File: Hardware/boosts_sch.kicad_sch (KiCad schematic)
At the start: 23 parts, among them IC3 AP2205-W5-7, IC4 TPS61089RNRR

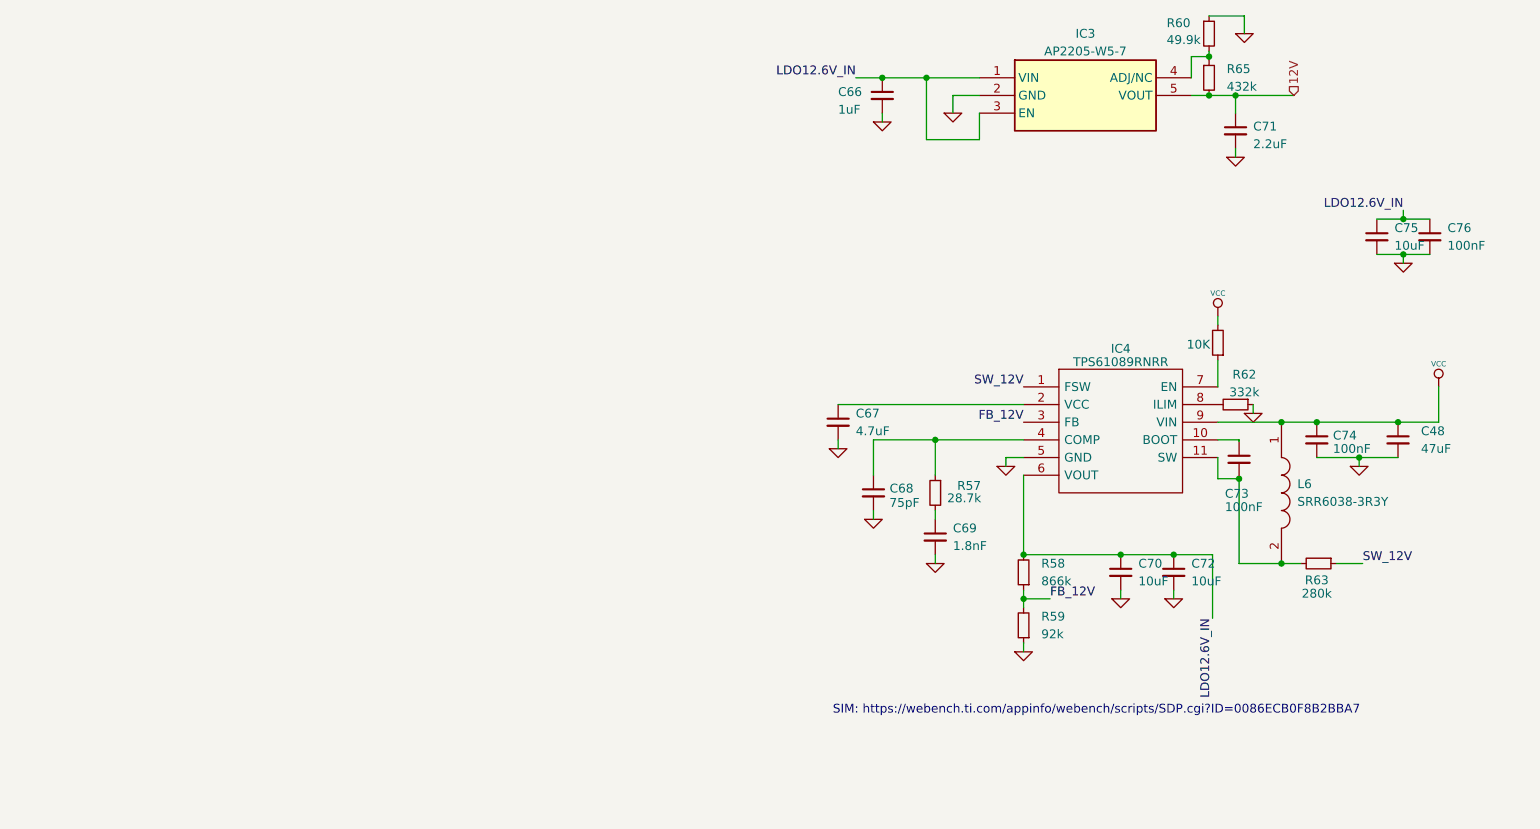
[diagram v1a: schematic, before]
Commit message: changes made post will's review
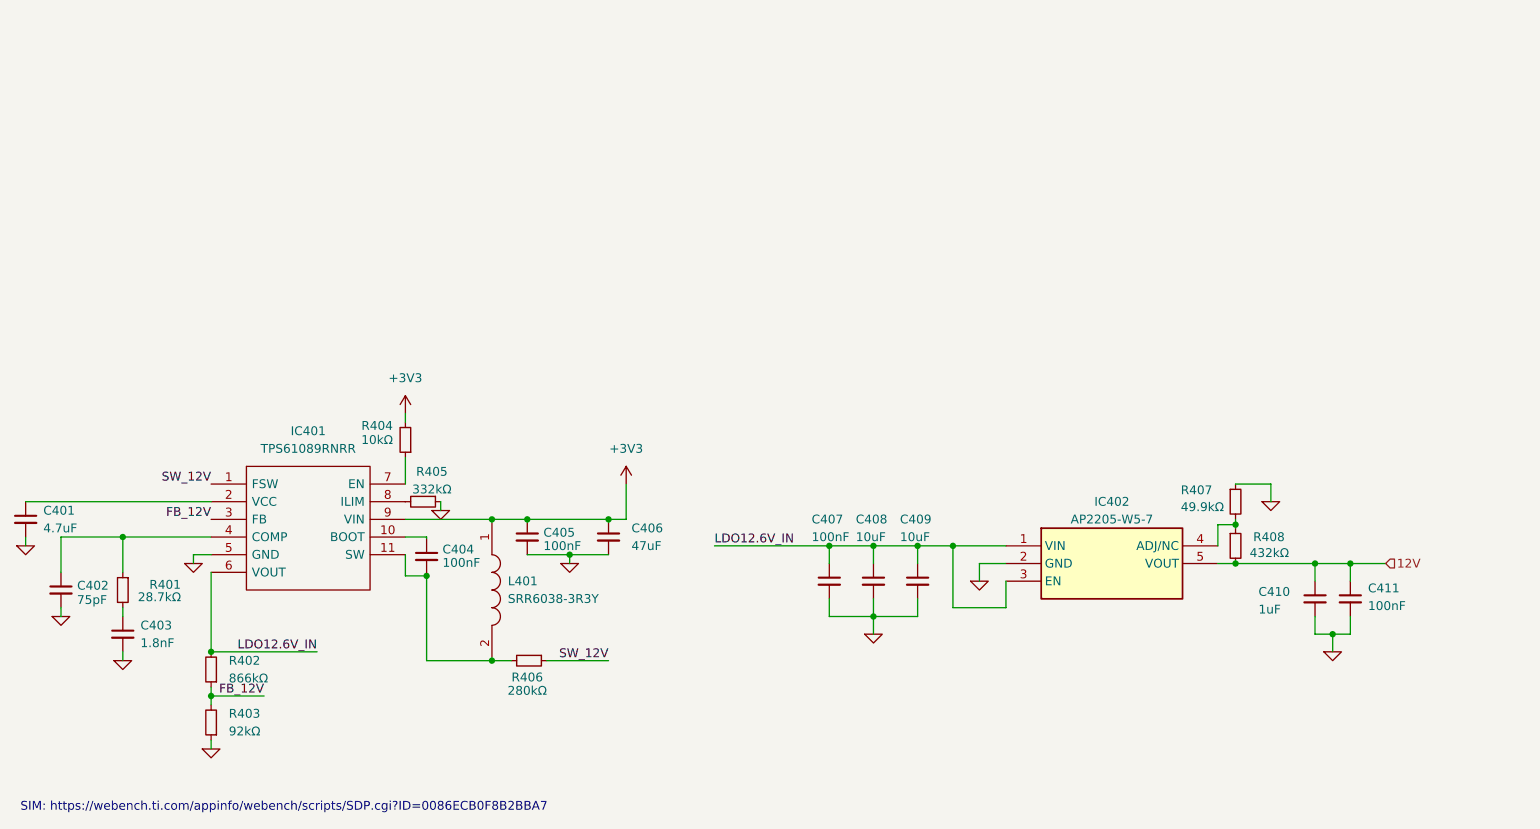
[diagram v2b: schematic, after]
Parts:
- removed C66: 1uF, Capacitor_SMD:C_0402_1005Metric, symbol Device:C_Small
- removed C70, C72: 10uF, Capacitor_SMD:C_0805_2012Metric, symbol Device:C_Small
- removed C71: 2.2uF, Capacitor_SMD:C_0402_1005Metric, symbol Device:C_Small
- removed C75: 10uF, Capacitor_SMD:C_0603_1608Metric, symbol Device:C_Small
- removed C76: 100nF, Capacitor_SMD:C_0402_1005Metric, symbol Device:C_Small
- added C407, C411: 100nF, Capacitor_SMD:C_0402_1005Metric, symbol Device:C_Small
- added C408, C409: 10uF, Capacitor_SMD:C_0805_2012Metric, symbol Device:C_Small
- added C410: 1uF, Capacitor_SMD:C_0603_1608Metric, symbol Device:C_Small
- R401: renamed from R57; value 28.7k -> 28.7kΩ
- R402: renamed from R58; value 866k -> 866kΩ
- R403: renamed from R59; value 92k -> 92kΩ
- R404: renamed from R61; value 10K -> 10kΩ
- R405: renamed from R62; value 332k -> 332kΩ
- R406: renamed from R63; value 280k -> 280kΩ
- R407: renamed from R60; value 49.9k -> 49.9kΩ
- R408: renamed from R65; value 432k -> 432kΩ
- renumbered C67 to C401, C68 to C402, C69 to C403, C73 to C404, C74 to C405, C48 to C406, IC4 to IC401, IC3 to IC402, L6 to L401
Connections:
- net 12V: now also C410.1, C411.1
- net GND: now also C407.2, C408.2, C409.2, C410.2, C411.2
- net LDO12.6V_IN: now also C407.1, C408.1, C409.1
- net VCC renamed +3V3
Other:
- moved on the sheet: C401, C402, C403, C404, C405, C406, IC401, IC402, L401, R401, R402, R403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
